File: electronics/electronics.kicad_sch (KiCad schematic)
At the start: 16 parts, among them J1 Barrel_Jack, J2 Conn_01x04_Pogo, J3 Conn_01x04_Pin, J4 Conn_01x04_Pin, U2 BA033CC0FP-E2, U3 ESP32-C6-MINI-1/U

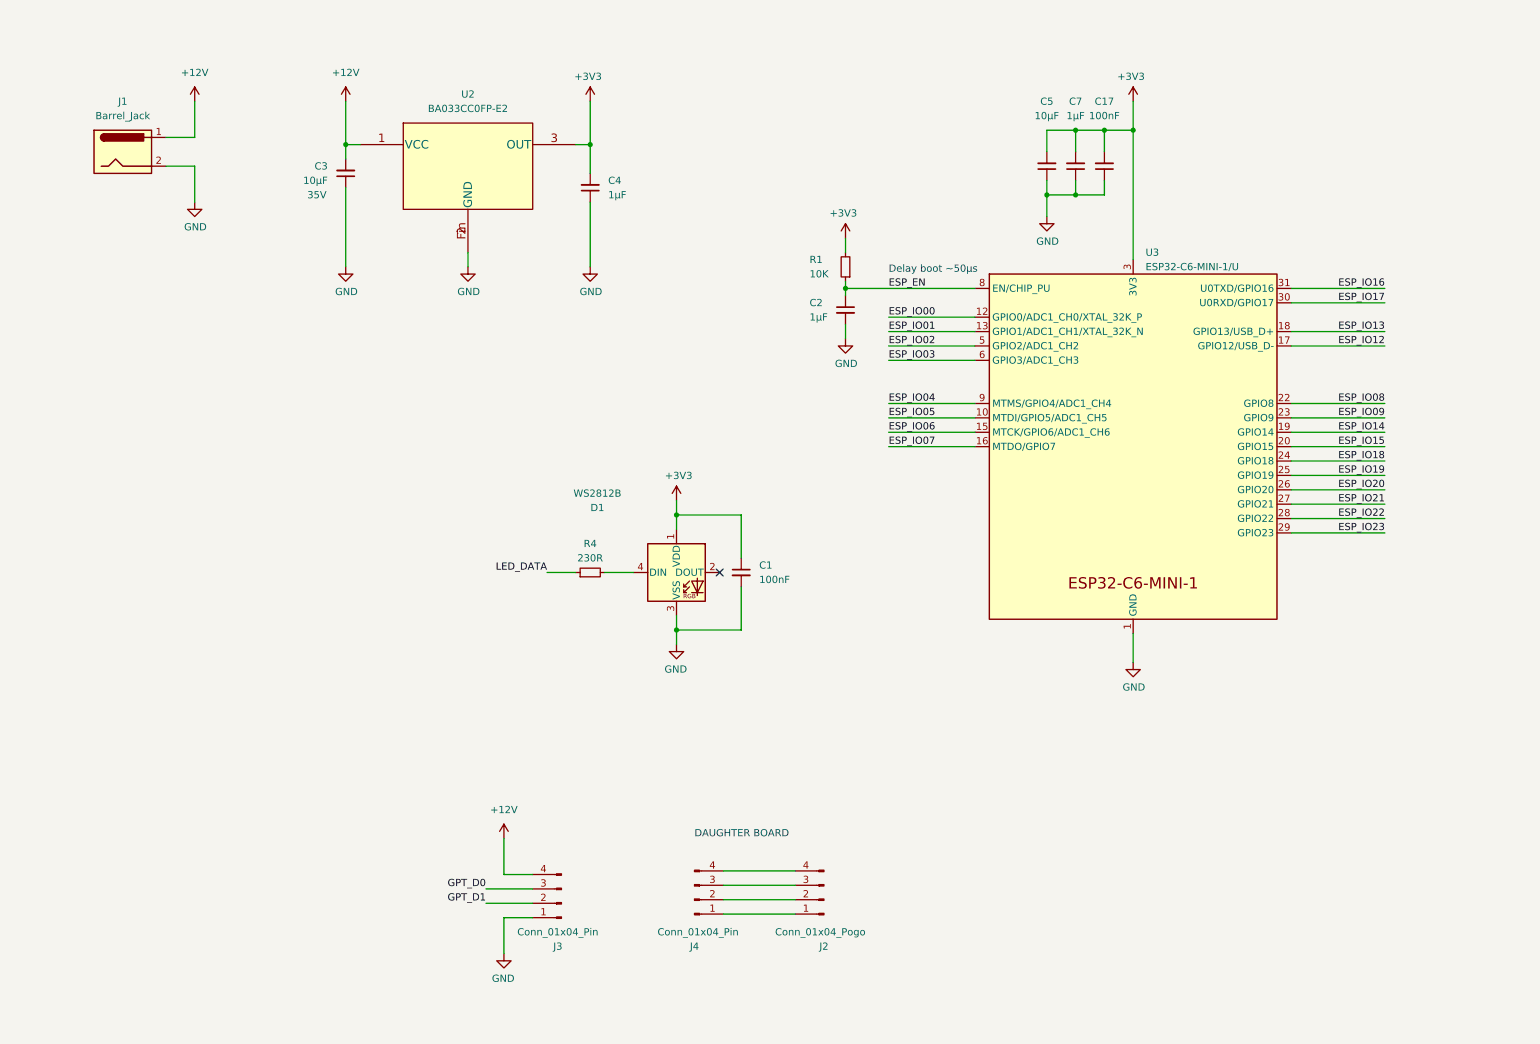
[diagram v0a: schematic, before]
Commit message: adding current prototypes
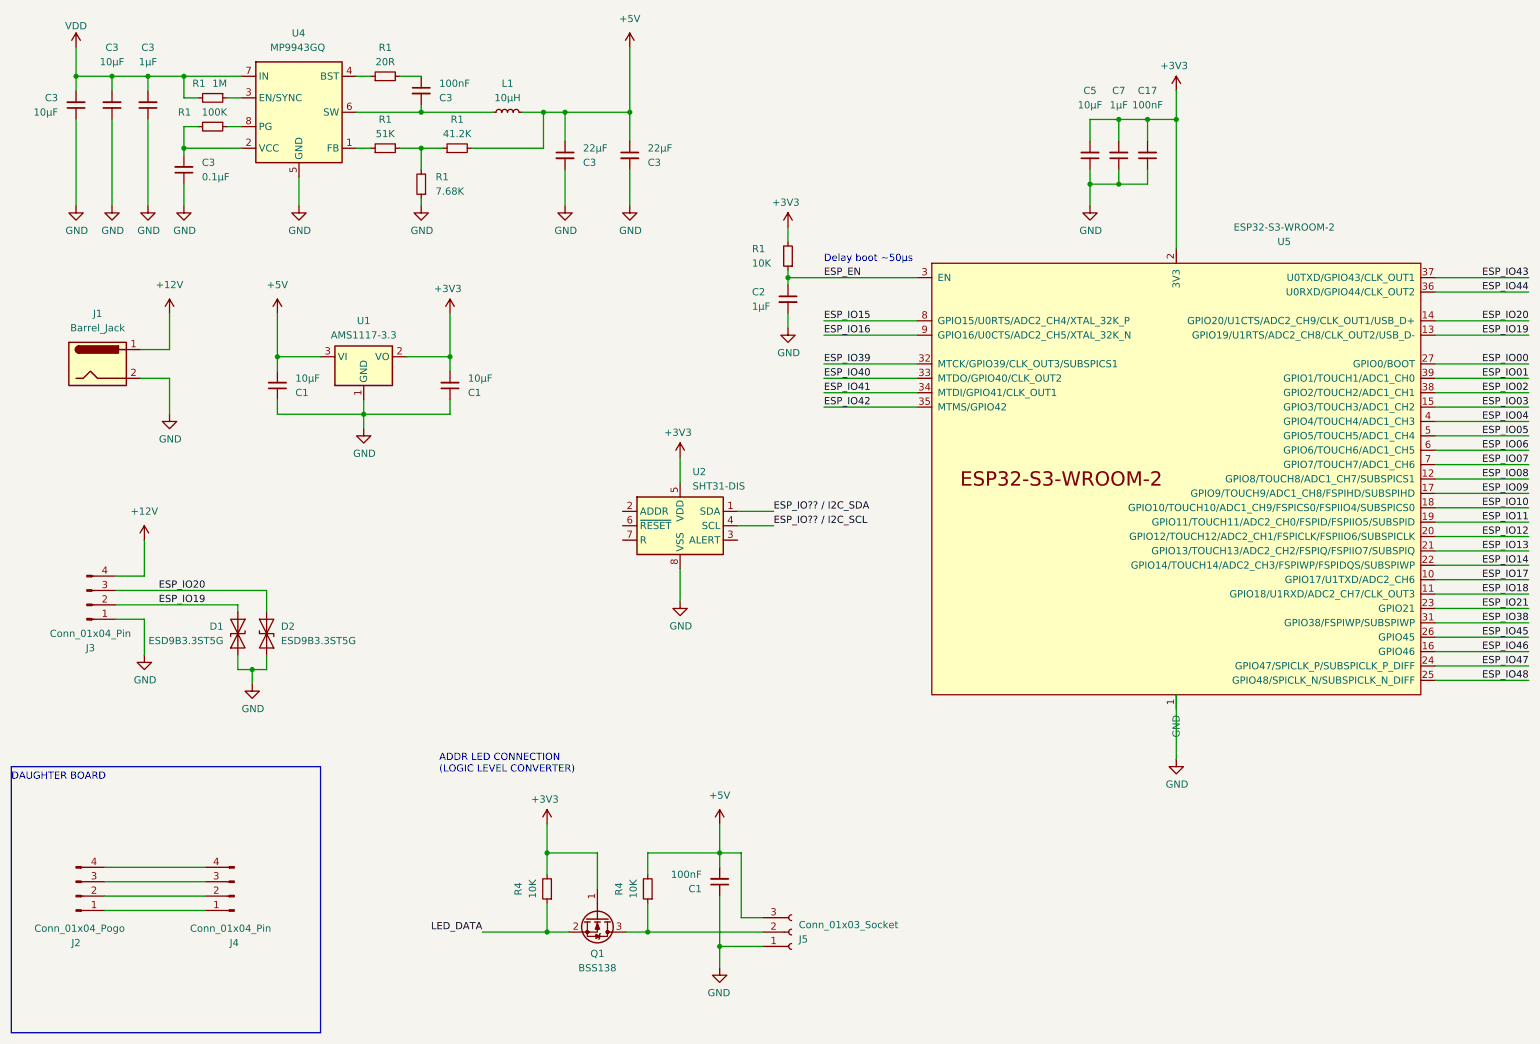
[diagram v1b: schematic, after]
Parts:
- removed C3: 10µF, Capacitor_SMD:C_0402_1005Metric, symbol Device:C_Small
- removed C4: 1µF, Capacitor_SMD:C_0402_1005Metric, symbol Device:C_Small
- removed D1: WS2812B, Slimc_LED_SMD:LED_WS2812C-2020, symbol LED:WS2812B
- removed R4: 230R, Resistor_SMD:R_0805_2012Metric_Pad1.20x1.40mm_HandSolder, symbol Device:R_Small
- removed U2: BA033CC0FP-E2, Package_TO_SOT_SMD:TO-252-2, symbol Slimc_Converter_DCDC:BAxxXX0
- removed U3: ESP32-C6-MINI-1/U, Espressif:ESP32-C6-MINI-1, symbol Espressif:ESP32-C6-MINI-1/U
- added C1 (x2), C3 (x2): 10µF, Capacitor_SMD:C_0402_1005Metric, symbol Device:C_Small
- added C3: 100nF, Capacitor_SMD:C_0402_1005Metric, symbol Device:C_Small
- added C3: 0.1µF, Capacitor_SMD:C_0402_1005Metric, symbol Device:C_Small
- added C3: 1µF, Capacitor_SMD:C_0402_1005Metric, symbol Device:C_Small
- added C3 (x2): 22µF, Capacitor_SMD:C_0402_1005Metric, symbol Device:C_Small
- added D1, D2: ESD9B3.3ST5G, Diode_SMD:D_SOD-923, symbol Diode:ESD9B3.3ST5G
- added J5: Conn_01x03_Socket, symbol Connector:Conn_01x03_Socket
- added L1: 10µH, symbol Device:L_Small
- added Q1: BSS138, Package_TO_SOT_SMD:SOT-23, symbol Transistor_FET:BSS138
- added R1: 1M, Resistor_SMD:R_0805_2012Metric_Pad1.20x1.40mm_HandSolder, symbol Device:R_Small
- added R1: 7.68K, Resistor_SMD:R_0805_2012Metric_Pad1.20x1.40mm_HandSolder, symbol Device:R_Small
- added R1: 20R, Resistor_SMD:R_0805_2012Metric_Pad1.20x1.40mm_HandSolder, symbol Device:R_Small
- added R1: 41.2K, Resistor_SMD:R_0805_2012Metric_Pad1.20x1.40mm_HandSolder, symbol Device:R_Small
- added R1: 51K, Resistor_SMD:R_0805_2012Metric_Pad1.20x1.40mm_HandSolder, symbol Device:R_Small
- added R1: 100K, Resistor_SMD:R_0805_2012Metric_Pad1.20x1.40mm_HandSolder, symbol Device:R_Small
- added R4 (x2): 10K, Resistor_SMD:R_0805_2012Metric_Pad1.20x1.40mm_HandSolder, symbol Device:R_Small
- added U1: AMS1117-3.3, Package_TO_SOT_SMD:SOT-223-3_TabPin2, symbol Regulator_Linear:AMS1117-3.3
- added U2: SHT31-DIS, Sensor_Humidity:Sensirion_DFN-8-1EP_2.5x2.5mm_P0.5mm_EP1.1x1.7mm, symbol Sensor_Humidity:SHT31-DIS
- added U4: MP9943GQ, Package_DFN_QFN:DFN-8-1EP_3x3mm_P0.65mm_EP1.7x2.05mm, symbol Slimc_Regulator_Switching:MP9943
- added U5: ESP32-S3-WROOM-2, Espressif:ESP32-S3-WROOM-2, symbol Espressif:ESP32-S3-WROOM-2
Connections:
- net GPT_D0 is gone; now on net ESP_IO20: J3.3 (Pin_3)
- net GPT_D1 is gone; now on net ESP_IO19: J3.2 (Pin_2)
- net +3V3: now also C1.2, Q1.1 (G), R4.2, U1.2 (VO), U2.5 (VDD), U5.2 (3V3); no longer C1.1
- net ESP_EN: now also U5.3 (EN)
- net ESP_IO00: now also U5.27 (GPIO0/BOOT)
- net ESP_IO01: now also U5.39 (GPIO1/TOUCH1/ADC1_CH0)
- net ESP_IO02: now also U5.38 (GPIO2/TOUCH2/ADC1_CH1)
- net ESP_IO03: now also U5.15 (GPIO3/TOUCH3/ADC1_CH2)
- net ESP_IO04: now also U5.4 (GPIO4/TOUCH4/ADC1_CH3)
- net ESP_IO05: now also U5.5 (GPIO5/TOUCH5/ADC1_CH4)
- net ESP_IO06: now also U5.6 (GPIO6/TOUCH6/ADC1_CH5)
- net ESP_IO07: now also U5.7 (GPIO7/TOUCH7/ADC1_CH6)
- net ESP_IO08: now also U5.12 (GPIO8/TOUCH8/ADC1_CH7/SUBSPICS1)
- net ESP_IO09: now also U5.17 (GPIO9/TOUCH9/ADC1_CH8/FSPIHD/SUBSPIHD)
- net ESP_IO12: now also U5.20 (GPIO12/TOUCH12/ADC2_CH1/FSPICLK/FSPIIO6/SUBSPICLK)
- net ESP_IO13: now also U5.21 (GPIO13/TOUCH13/ADC2_CH2/FSPIQ/FSPIIO7/SUBSPIQ)
- net ESP_IO14: now also U5.22 (GPIO14/TOUCH14/ADC2_CH3/FSPIWP/FSPIDQS/SUBSPIWP)
- net ESP_IO15: now also U5.8 (GPIO15/U0RTS/ADC2_CH4/XTAL_32K_P)
- net ESP_IO16: now also U5.9 (GPIO16/U0CTS/ADC2_CH5/XTAL_32K_N)
- net ESP_IO17: now also U5.10 (GPIO17/U1TXD/ADC2_CH6)
- net ESP_IO18: now also U5.11 (GPIO18/U1RXD/ADC2_CH7/CLK_OUT3)
- net ESP_IO19: now also D1.1 (A1), U5.13 (GPIO19/U1RTS/ADC2_CH8/CLK_OUT2/USB_D-)
- net ESP_IO20: now also D2.1 (A1), U5.14 (GPIO20/U1CTS/ADC2_CH9/CLK_OUT1/USB_D+)
- net ESP_IO21: now also U5.23 (GPIO21)
- net GND: now also C1.1, C1.1, C1.1, C3.1, C3.1, C3.1, C3.1, C3.2, C3.2, D1.2 (A2), D2.2 (A2), J5.1 (Pin_1), R1.1, U1.1 (GND), U2.8 (VSS), U2.9 (VSS), U4.5 (GND), U5.1 (GND), U5.40 (GND), U5.41 (GND); no longer C1.2
- net LED_DATA: now also Q1.2 (S), R4.1
- new net: C3.1, R1.2
- new net: C3.2, L1.1, U4.6 (SW)
- new net: R1.1, U4.3 (EN/SYNC)
- new net: J5.2 (Pin_2), Q1.3 (D), R4.1
- new net: C3.2, R1.2, U4.2 (VCC)
- new net: R1.1, R1.2, R1.2
- new net: R1.1, U4.4 (BST)
- new net: R1.1, U4.1 (FB)
- new net: R1.1, U4.8 (PG)
- new net +5V: C1.2, C1.2, C3.1, C3.1, J5.3 (Pin_3), L1.2, R1.2, R4.2, U1.3 (VI)
- new net ESP_IO10: U5.18 (GPIO10/TOUCH10/ADC1_CH9/FSPICS0/FSPIIO4/SUBSPICS0)
- new net ESP_IO11: U5.19 (GPIO11/TOUCH11/ADC2_CH0/FSPID/FSPIIO5/SUBSPID)
- new net ESP_IO38: U5.31 (GPIO38/FSPIWP/SUBSPIWP)
- new net ESP_IO39: U5.32 (MTCK/GPIO39/CLK_OUT3/SUBSPICS1)
- new net ESP_IO40: U5.33 (MTDO/GPIO40/CLK_OUT2)
- new net ESP_IO41: U5.34 (MTDI/GPIO41/CLK_OUT1)
- new net ESP_IO42: U5.35 (MTMS/GPIO42)
- new net ESP_IO43: U5.37 (U0TXD/GPIO43/CLK_OUT1)
- new net ESP_IO44: U5.36 (U0RXD/GPIO44/CLK_OUT2)
- new net ESP_IO45: U5.26 (GPIO45)
- new net ESP_IO46: U5.16 (GPIO46)
- new net ESP_IO47: U5.24 (GPIO47/SPICLK_P/SUBSPICLK_P_DIFF)
- new net ESP_IO48: U5.25 (GPIO48/SPICLK_N/SUBSPICLK_N_DIFF)
- new net ESP_IO?? / I2C_SCL: U2.4 (SCL)
- new net ESP_IO?? / I2C_SDA: U2.1 (SDA)
- new net VDD: C3.2, C3.2, C3.2, R1.2, U4.7 (IN)
- no-connect marks 1 -> 0
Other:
- note added: "ADDR LED CONNECTION (LOGIC LEVEL CONVERTER)"
- moved on the sheet: C1, C17, C2, C5, C7, J1, J2, J3, J4, R1
